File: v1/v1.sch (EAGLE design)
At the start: 19 parts, among them J1 ATX24RH, J2 24VAC, Q1 TIP120, Q2 TIP120, Q3 TIP120, Q4 TIP120, Q5 TIP120, Q6 TIP120, U1 ARDUINO-MEGAFULL

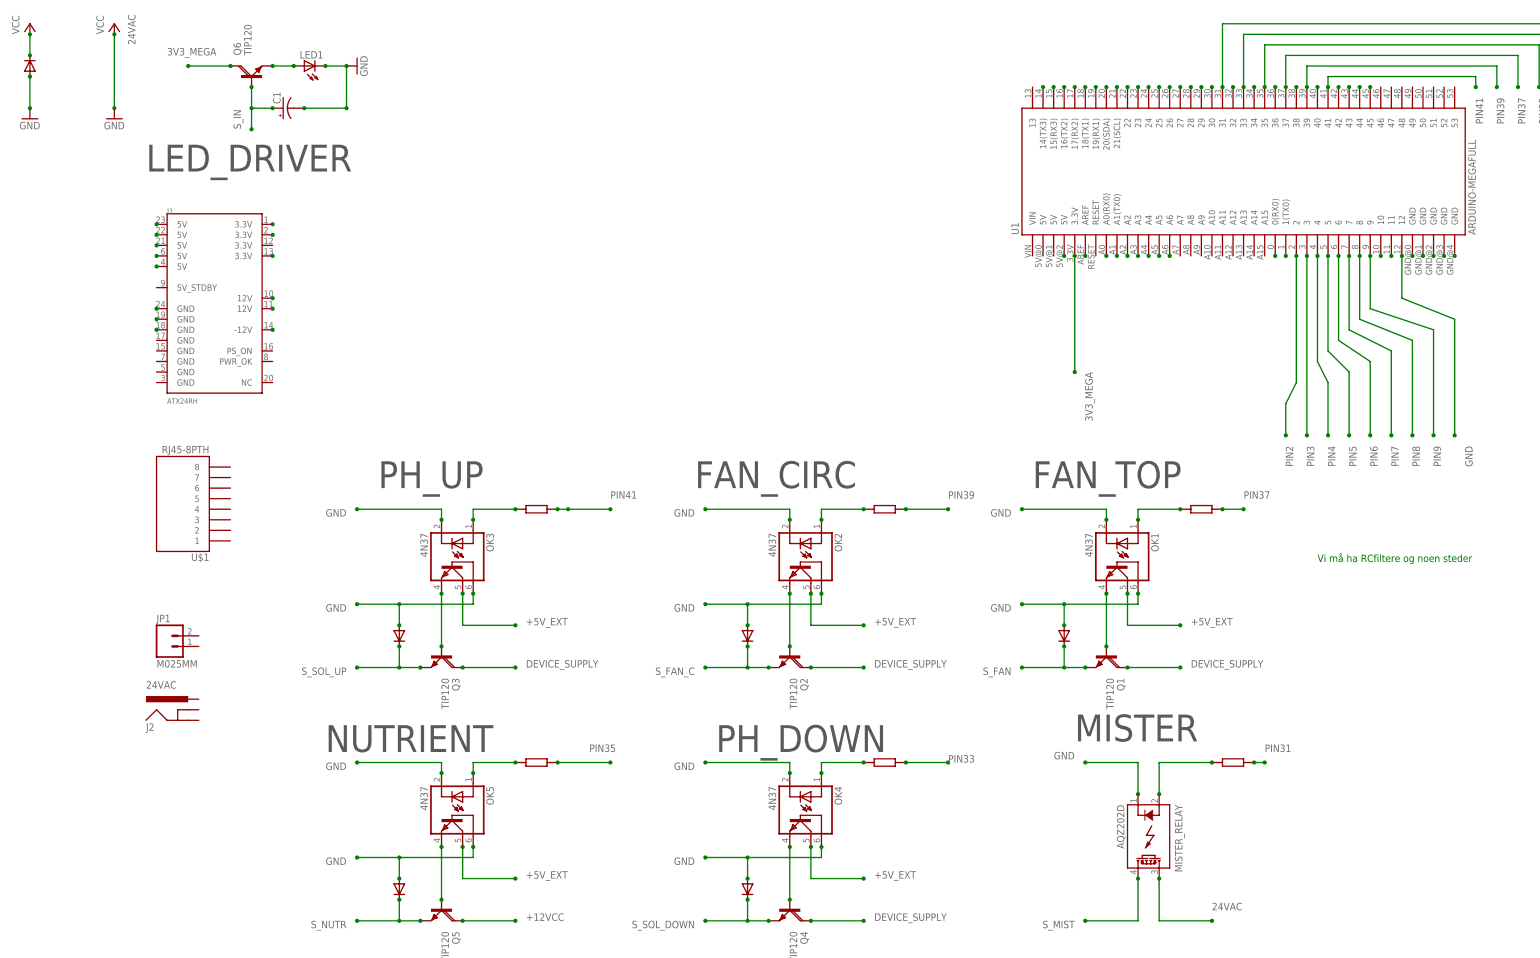
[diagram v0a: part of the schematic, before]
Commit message: last
more changes to come
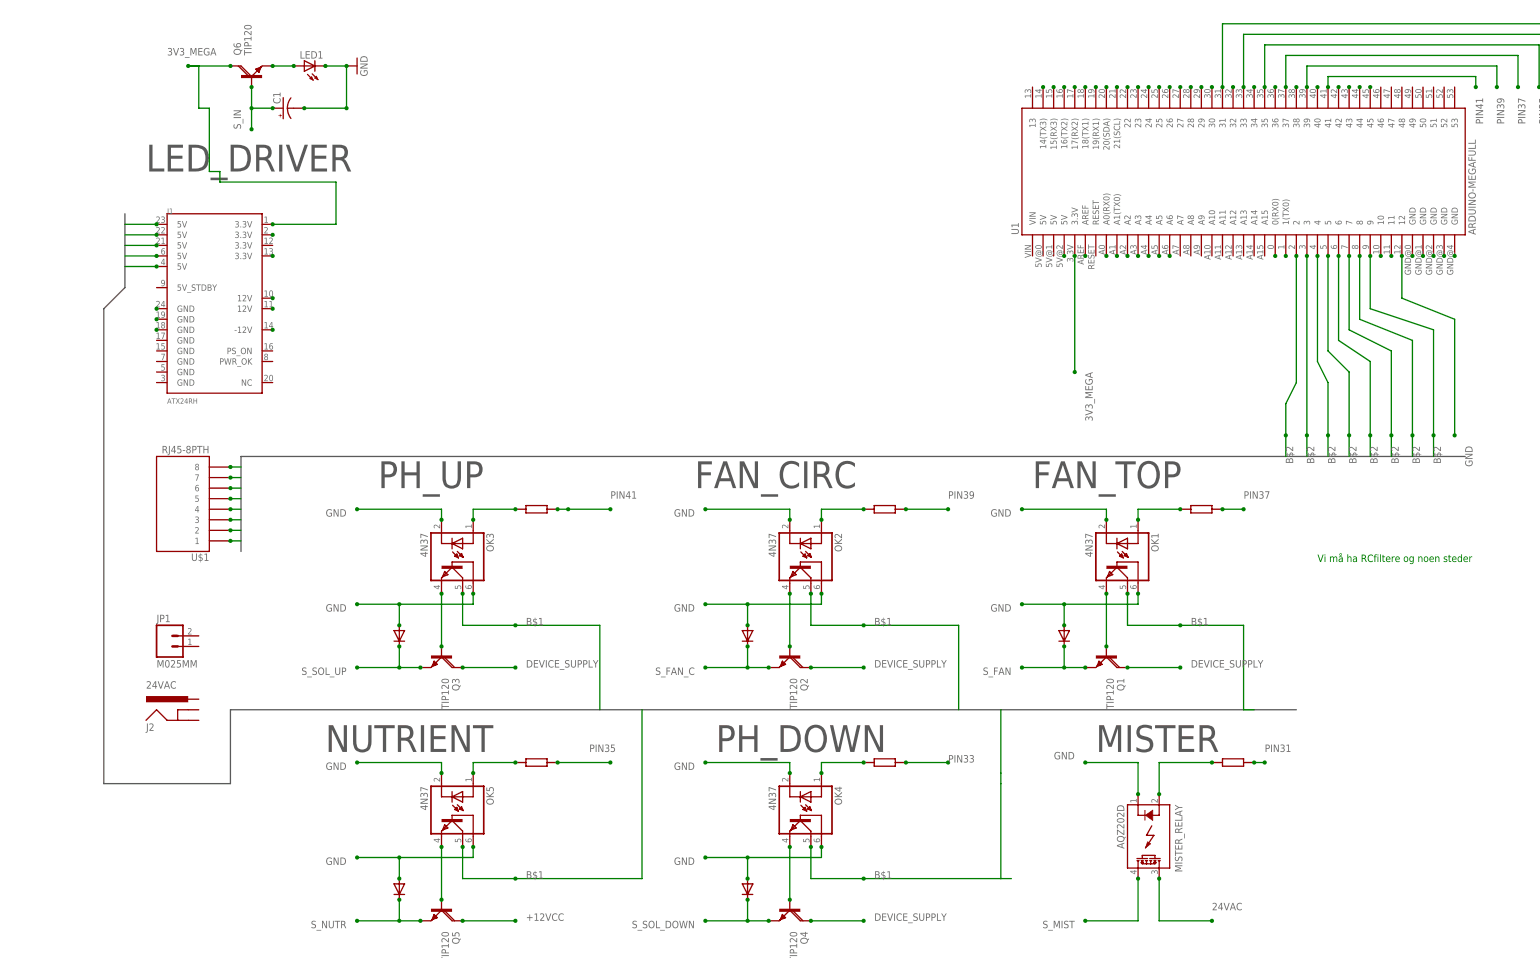
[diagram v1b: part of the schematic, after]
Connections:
- removed net +5V_EXT: OK1.COL, OK2.COL, OK3.COL, OK4.COL, OK5.COL
- removed net N$19: J1.5V@4
- removed net N$29: J1.5V@3
- removed net N$56: J1.5V@2
- removed net N$57: J1.5V@0
- removed net N$58: J1.5V@1
- removed net N$59: J1.3.3V@0
- removed net PIN2: U1.2
- removed net PIN3: U1.3
- removed net PIN4: U1.4
- removed net PIN5: U1.5
- removed net PIN6: U1.6
- removed net PIN7: U1.7
- removed net PIN8: U1.8
- removed net PIN9: U1.9
- new net B$1: J1.5V@0, J1.5V@1, J1.5V@2, J1.5V@3, J1.5V@4, OK1.COL, OK2.COL, OK3.COL, OK4.COL, OK5.COL
- new net B$2: U$1.1, U$1.2, U$1.3, U$1.4, U$1.5, U$1.6, U$1.7, U$1.8, U1.2, U1.3, U1.4, U1.5, U1.6, U1.7, U1.8, U1.9
- net 3V3_MEGA: now also J1.3.3V@0
